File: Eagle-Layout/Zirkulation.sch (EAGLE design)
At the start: 13 parts, among them X1 MKDSN1,5/3-5,08

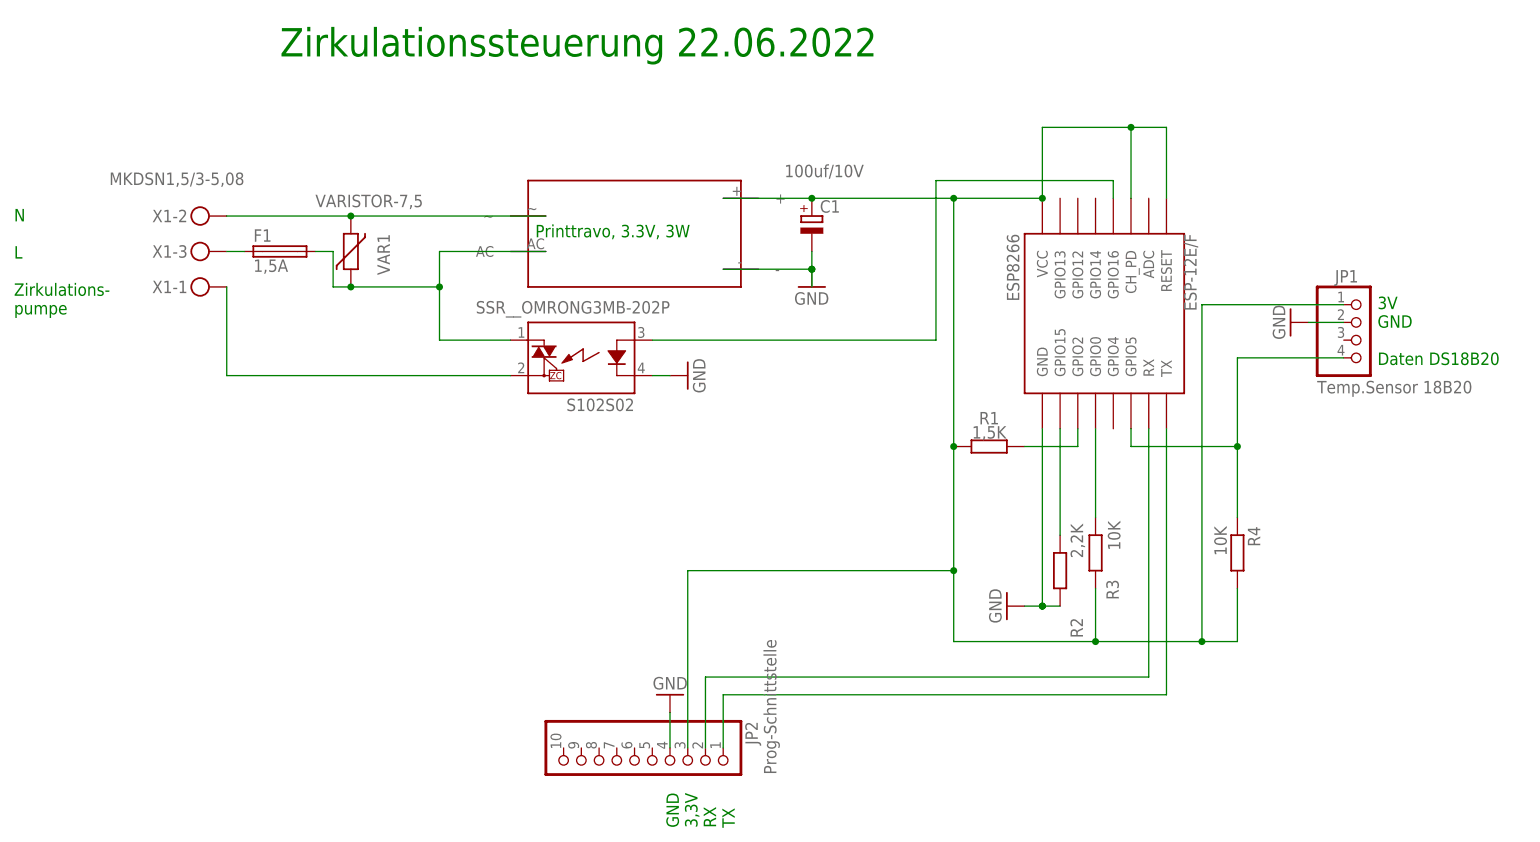
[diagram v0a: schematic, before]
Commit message: Personal custom variant of Heise Zirkulationspumpe
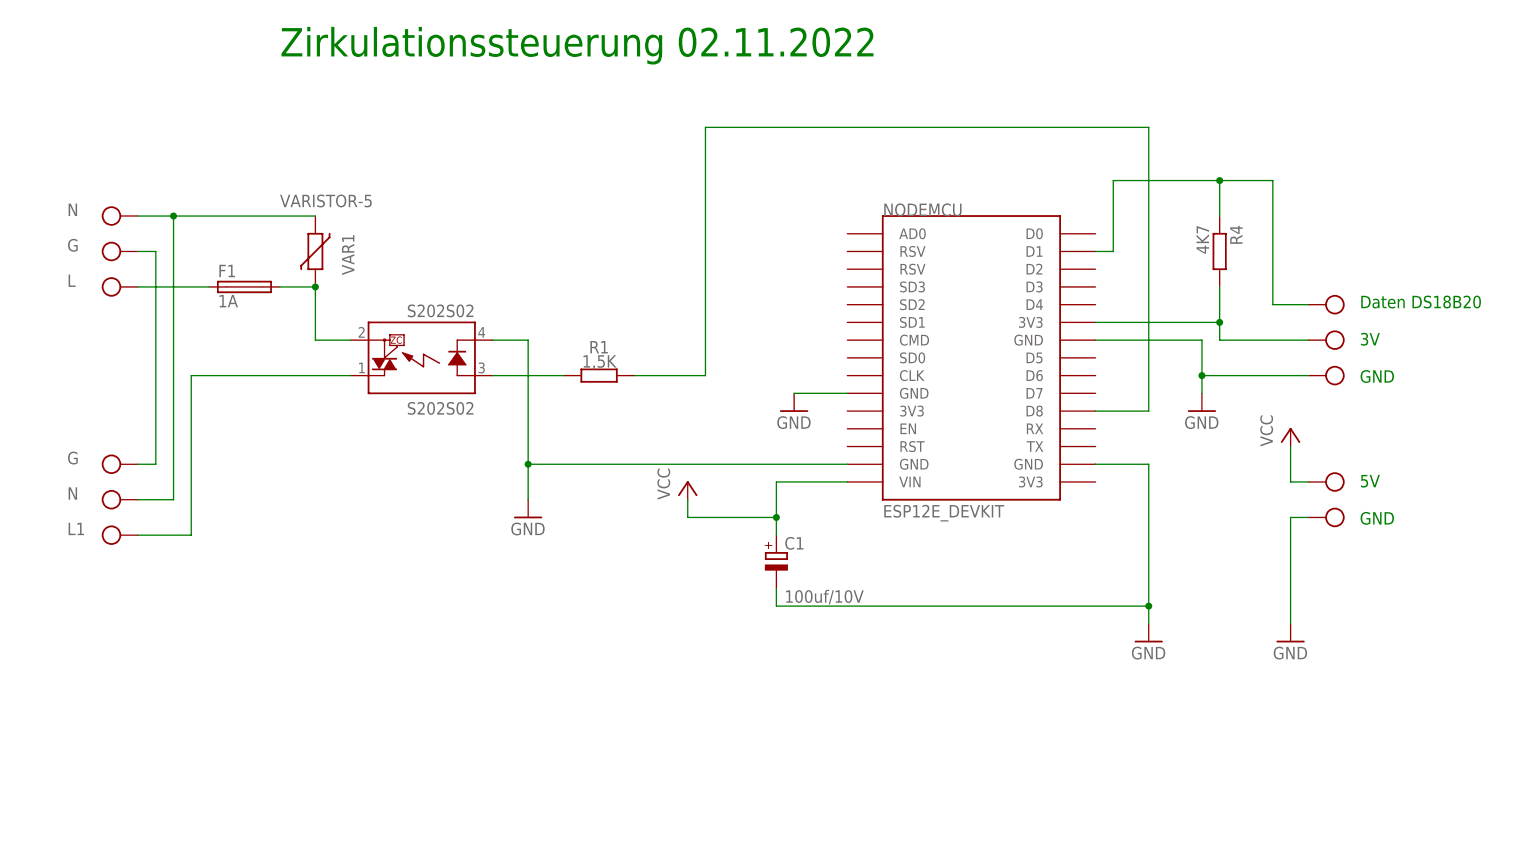
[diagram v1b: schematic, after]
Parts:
- removed ESP-12E/F: ESP8266, esp8266modules:ESP12SMD
- removed JP1: Temp.Sensor 18B20, pinhead:PINHD-1X4
- removed JP2: Prog-Schnittstelle, pinhead:PINHD-1X10
- removed PRINTTRAFO3.3V,_3W: PRINTTRAFO, Uwes_lib:PRINTTRAFO
- removed R2: 2,2K, rcl:R-EU_0204/7
- removed R3: 10K, rcl:R-EU_0204/7
- removed SSR__OMRONG3MB-202P: S102S02, relay:S102S02
- removed X1: MKDSN1,5/3-5,08, con-phoenix-508:MKDSN1,5/3-5,08
- added IN, OUT, SENSOR: MKDSN1,5/3-5,08, my_con-phoenix-508:MKDSN1,5/3-5,08
- added NODEMCU: ESP12E_DEVKIT, ESP12E_DEVKIT:ESP12E_DEVKIT
- added PWR: MKDSN1,5/2-5,08, my_con-phoenix-508:MKDSN1,5/2-5,08
- added S202S02: S202S02, my_relay:S202S02
- C1: device rcl:CPOL-EUE2.5-7 -> my_rcl:CPOL-EUE2.5-7
- F1: value 1,5A -> 1A; device fuse:LITTLEFUSE -> my_fuse:FUSESH22,5
- R1: device rcl:R-EU_0204/7 -> my_rcl:R-EU_0204/5
- R4: value 10K -> 4K7; device rcl:R-EU_0204/7 -> my_rcl:R-EU_0204/5
- VAR1: value VARISTOR-7,5 -> VARISTOR-5; device varistor:VARISTOR-7,5 -> my_varistor:VARISTOR-5
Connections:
- removed net 3.3V: C1.+, ESP-12E/F.CH_PD, ESP-12E/F.RESET, ESP-12E/F.VCC, JP1.1, JP2.3, PRINTTRAFO3.3V,_3W.+, R1.2, R3.2, R4.2
- removed net GPIO0: ESP-12E/F.GPIO0, R3.1
- removed net GPIO15: ESP-12E/F.GPIO15, R2.2
- removed net GPIO16: ESP-12E/F.GPIO16, SSR__OMRONG3MB-202P.A
- removed net GPIO2: ESP-12E/F.GPIO2, R1.1
- removed net GPIO5: ESP-12E/F.GPIO5, JP1.4, R4.1
- removed net L_: F1.2, PRINTTRAFO3.3V,_3W.AC, SSR__OMRONG3MB-202P.DS1, VAR1.1
- removed net RX: ESP-12E/F.RX, JP2.2
- removed net TX: ESP-12E/F.TX, JP2.1
- new net G: IN-3.KL, OUT-3.KL
- new net LF: F1.2, S202S02.DS2, VAR1.1
- new net N$2: R1.2, S202S02.A
- new net N$5: NODEMCU.D8, R1.1
- new net N$6: NODEMCU.3V3@1, R4.2, SENSOR-2.KL
- new net N$7: NODEMCU.D1, R4.1, SENSOR-1.KL
- new net VCC: C1.+, NODEMCU.VIN, PWR-1.KL
- net GND: now also NODEMCU.GND@0, NODEMCU.GND@1, NODEMCU.GND@2, NODEMCU.GND@3, PWR-2.KL, S202S02.K, SENSOR-3.KL; no longer ESP-12E/F.GND, JP1.2, JP2.4, PRINTTRAFO3.3V,_3W.-, R2.1, SSR__OMRONG3MB-202P.K
- net L: now also IN-1.KL; no longer X1-3.KL
- net L1: now also OUT-1.KL, S202S02.DS1; no longer SSR__OMRONG3MB-202P.DS2, X1-1.KL
- net N: now also IN-2.KL, OUT-2.KL; no longer PRINTTRAFO3.3V,_3W.~, X1-2.KL
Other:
- note added: "5V GND"
- note added: "Daten DS18B20 3V GND"
- note added: "Zirkulationssteuerung 02.11.2022"
- note removed: "3V GND Daten DS18B20"
- note removed: "GND 3,3V RX TX"
- note removed: "N L Zirkulations- pumpe"
- note removed: "Printtravo, 3.3V, 3W"
- note removed: "Zirkulationssteuerung 22.06.2022"
- moved on the sheet: C1, R1, R4, VAR1
